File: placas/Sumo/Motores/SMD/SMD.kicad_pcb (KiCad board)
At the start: 2 copper layers, 46.2 x 25.3 mm, 5 parts, among them J1 DATOS, J2 ALIMENTACION, J3 MOTORES, U1 VNH3SP30

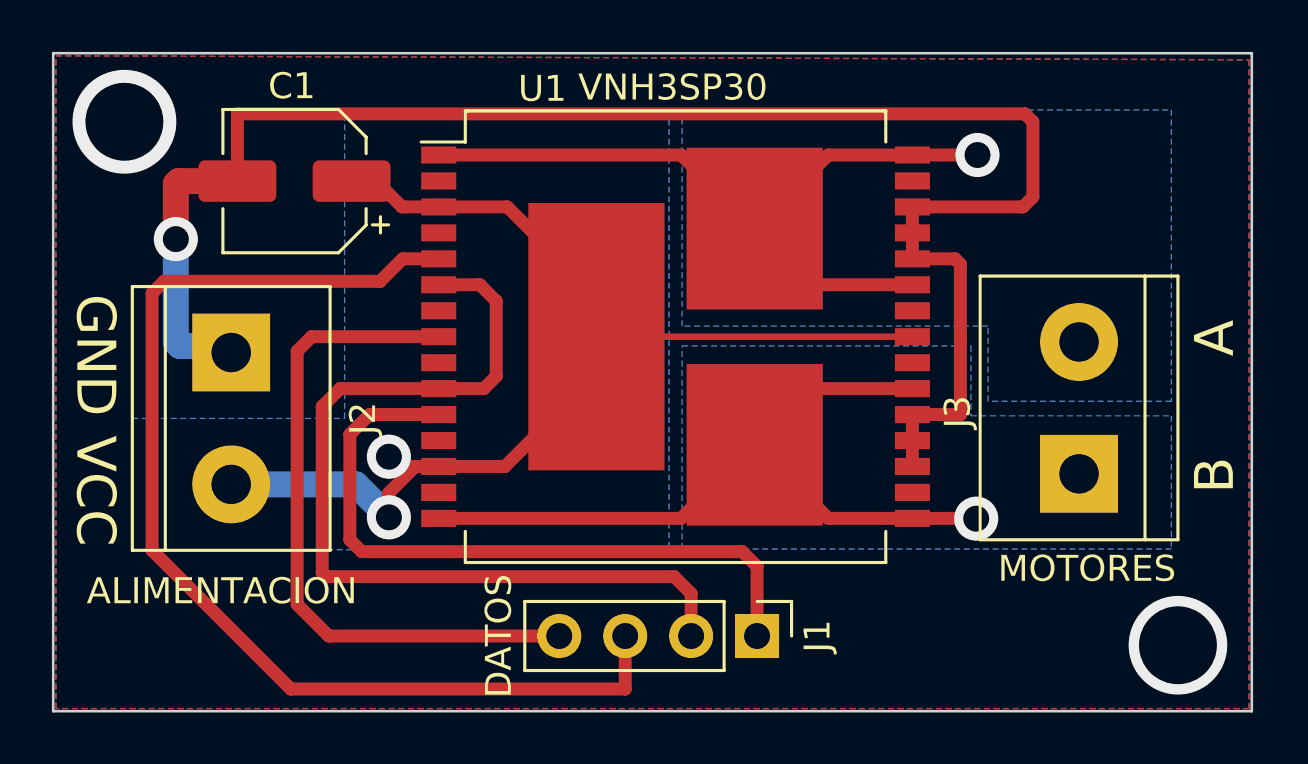
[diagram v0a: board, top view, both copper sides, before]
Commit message: wed
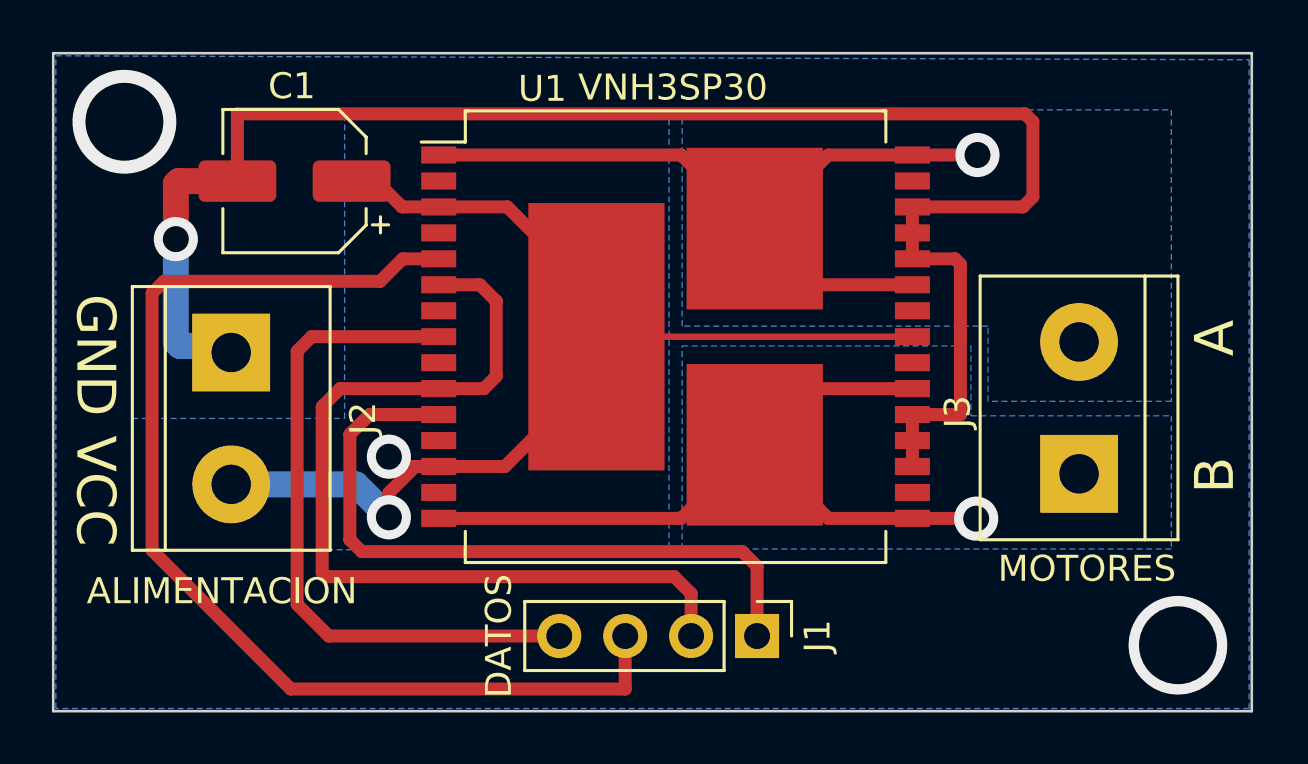
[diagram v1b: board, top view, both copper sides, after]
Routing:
- removed copper zone on F.Cu, net GND
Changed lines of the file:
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@@
   (segment (start 12.2936 34.3916) (end 12.5476 34.6456) (width 1) (layer "B.Cu") (net 15))
   (segment (start 13.1064 34.3916) (end 10.5664 34.3916) (width 1) (layer "B.Cu") (net 15))
-  (zone (net 15) (net_name "GND") (layers F&B.Cu) (hatch edge 0.508)
-    (connect_pads (clearance 0.508))
-    (min_thickness 0.254) (filled_areas_thickness no)
-    (fill yes (thermal_gap 0.508) (thermal_bridge_width 0.508))
-    (polygon
-      (pts
-        (xy 51.7652 48.3616)
-        (xy 5.7912 48.3616)
-        (xy 5.7912 23.2156)
-        (xy 51.7652 23.368)
-      )
-    )
-  )
   (zone (net 13) (net_name "/OUTB") (layer "B.Cu") (hatch edge 0.508)
     (priority 1)
@@
       )
     )
+  )
+  (zone (net 15) (net_name "GND") (layer "B.Cu") (hatch edge 0.508)
+    (connect_pads (clearance 0.508))
+    (min_thickness 0.254) (filled_areas_thickness no)
+    (fill yes (thermal_gap 0.508) (thermal_bridge_width 0.508))
+    (polygon
+      (pts
+        (xy 51.7652 48.3616)
+        (xy 5.7912 48.3616)
+        (xy 5.7912 23.2156)
+        (xy 51.7652 23.368)
+      )
+    )
